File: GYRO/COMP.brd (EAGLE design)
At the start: 57.1 x 32.7 mm, 59 parts, among them J10 SM02B-SRSS-TB(LF)(SN), J11 47346-0001, J12 EVP-ANDA1A, J13 EVP-ANDA1A, J14 EVP-ANDA1A, J15 EVP-ANDA1A, J3 PIN_1X.1", J4 PIN_1X.1", J5 PIN_1X.1", J6 PIN_1X.1", J7 PIN_1X.1", J8 PIN_1X.1", Q1 DMP2035U, SW1 PCM12SMTR, U1 XC6210B33, U2 TX0102, U3 MCP73831, U4 L3G4200D, U5 ATSAMD21G18A, U6 XC6210B33, U7 UG-9664HDDAG01, U8 FAN5340, Y1 32.7680

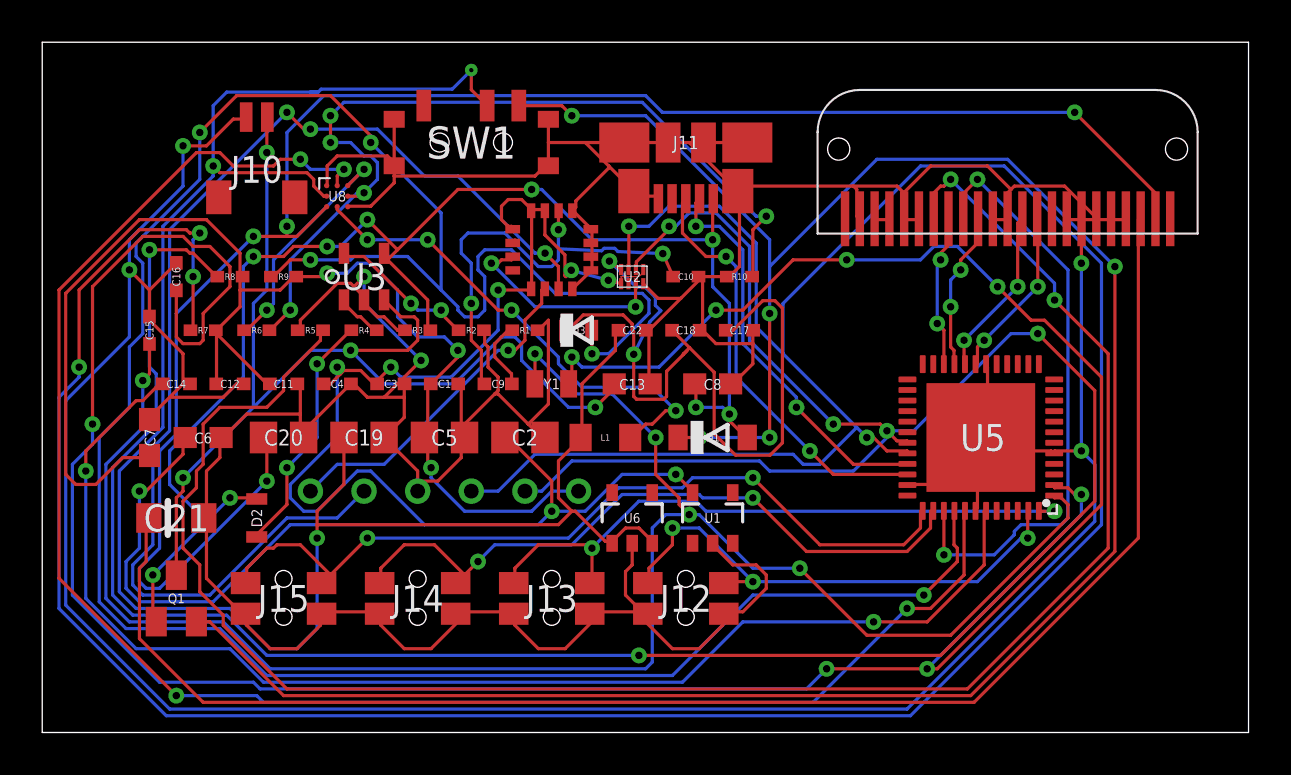
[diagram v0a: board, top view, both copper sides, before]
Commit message: sd
sd
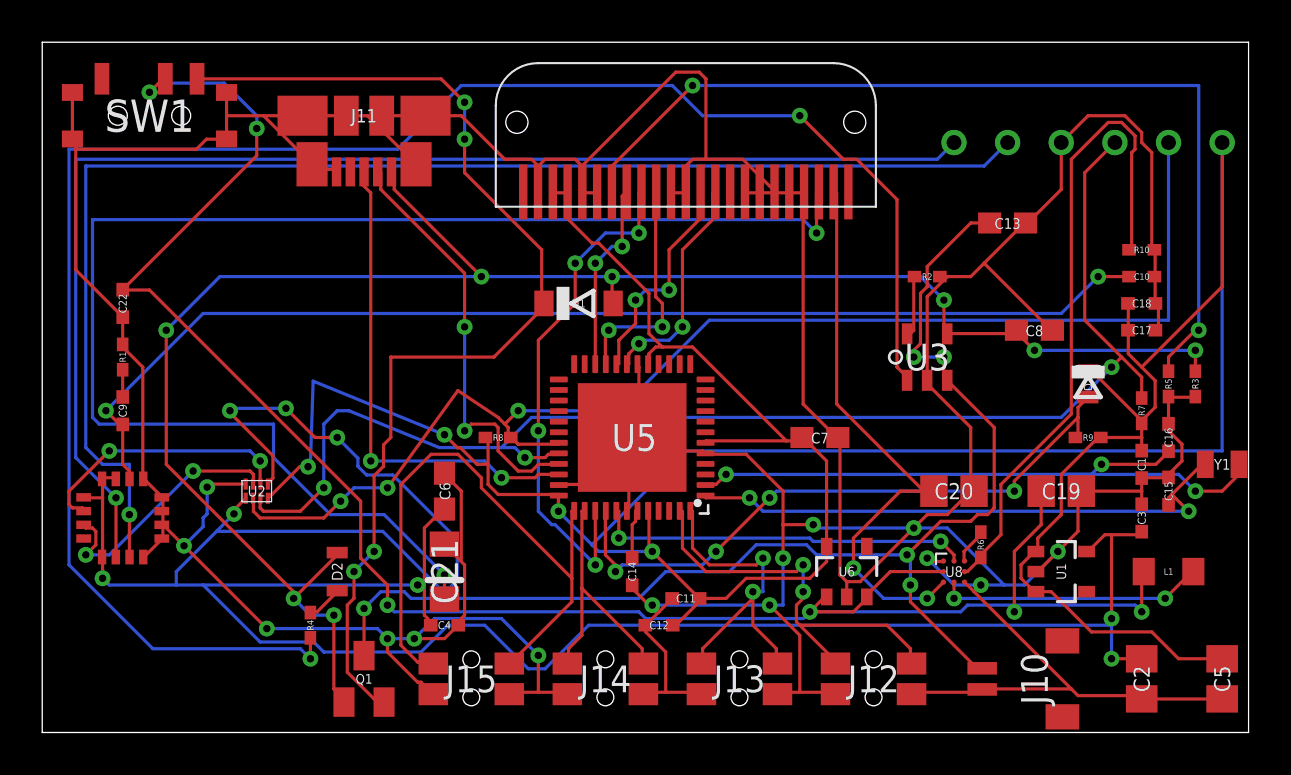
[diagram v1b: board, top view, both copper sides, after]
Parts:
- moved C15 48.9 mm to (90.2, 80.0)
- moved C16 47.6 mm to (90.2, 82.5)
- moved R7 44.6 mm to (88.9, 83.8), turned to 270 degrees
- moved J10 44.0 mm to (83.8, 71.1), turned to 90 degrees
- moved R5 40.7 mm to (90.2, 85.1), turned to 90 degrees
- moved R9 38.9 mm to (86.4, 82.5)
- moved C5 38.6 mm to (92.7, 71.1), turned to 270 degrees
- moved R3 36.9 mm to (91.4, 85.1), turned to 90 degrees
- moved C3 36.1 mm to (88.9, 78.7), turned to 90 degrees
- moved R6 35.8 mm to (81.3, 77.5), turned to 270 degrees
- moved J4 34.7 mm to (90.2, 96.5)
- moved J6 34.7 mm to (85.1, 96.5)
- moved J8 34.7 mm to (80.0, 96.5)
- moved J3 34.7 mm to (92.7, 96.5)
- moved J5 34.7 mm to (87.6, 96.5)
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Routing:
- net N$8: track 135.5 -> 32.6 mm, vias 8 -> 3
- net AD5/SCL: track 159.7 -> 64.0 mm, vias 5 -> 3
- net RESET: track 118.6 -> 30.5 mm, vias 5 -> 4
- net N$7: track 2.33 -> 85.4 mm, vias 0 -> 2
- net AD4/SDA: track 130.3 -> 61.3 mm, vias 6 -> 3
- net USB_HOST_EN/IO27: track 82.2 -> 17.9 mm, vias 4 -> 2
- net VCC: track 101.2 -> 163.8 mm, vias 5 -> 4
- net N$3: track 110.0 -> 50.8 mm, vias 5 -> 4
- net N$4: track 85.9 -> 27.1 mm, vias 5 -> 2
- net N$9: track 61.1 -> 2.37 mm, vias 2 -> 0
- net +12V: track 83.1 -> 27.4 mm, vias 4 -> 2
- net INT2: track 16.0 -> 61.5 mm
- net N$11: track 87.6 -> 44.8 mm
- net VCC_3V3: track 88.3 -> 122.9 mm
- net N$2: track 21.5 -> 54.9 mm, vias 3 -> 2
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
